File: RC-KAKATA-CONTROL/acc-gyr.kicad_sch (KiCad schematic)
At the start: 10 parts, among them U13 ICM-20689

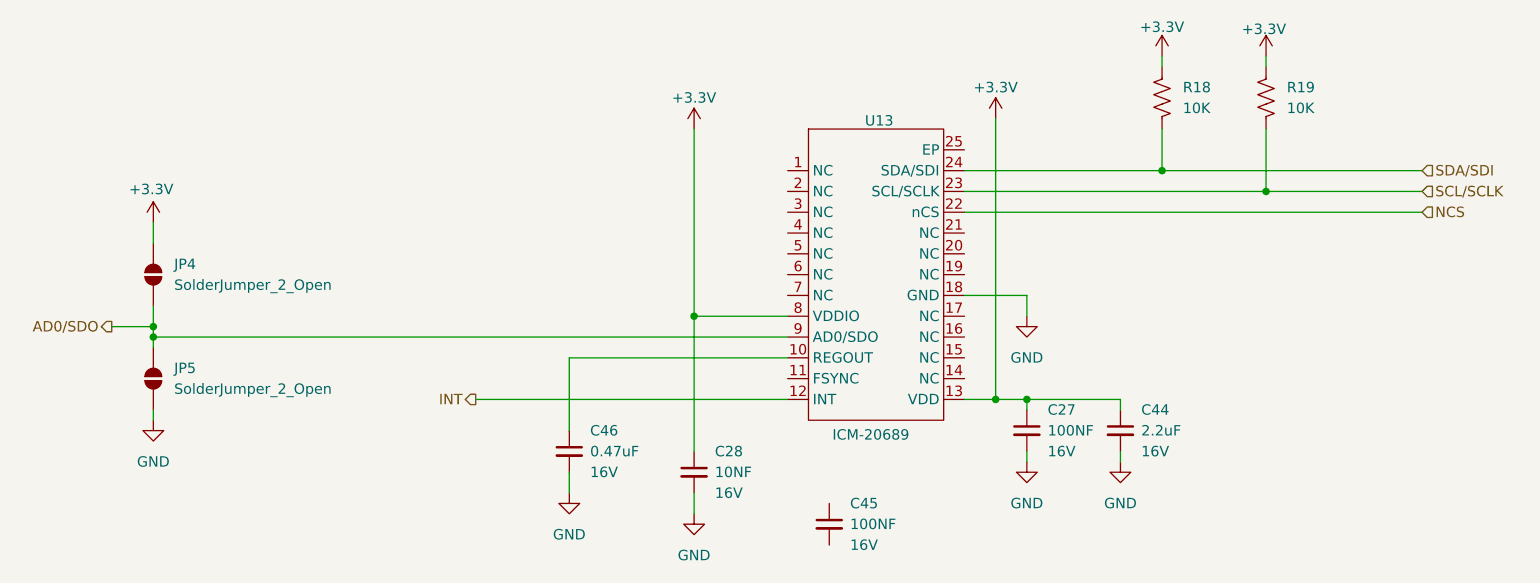
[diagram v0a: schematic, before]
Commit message: Agregadas conexiones de analogicos Agregadas las conexiones de i2c Agregadas las conexiones de Uart Cambiados algunos detalles de tvs resistencias y cap Recolocados los componenetes de power supply Cambiados los diodos de entrada de la bateria por unos de 5A Cambios menores y mejorada la documentacion Agregada informacion en la serigrafia del PCB
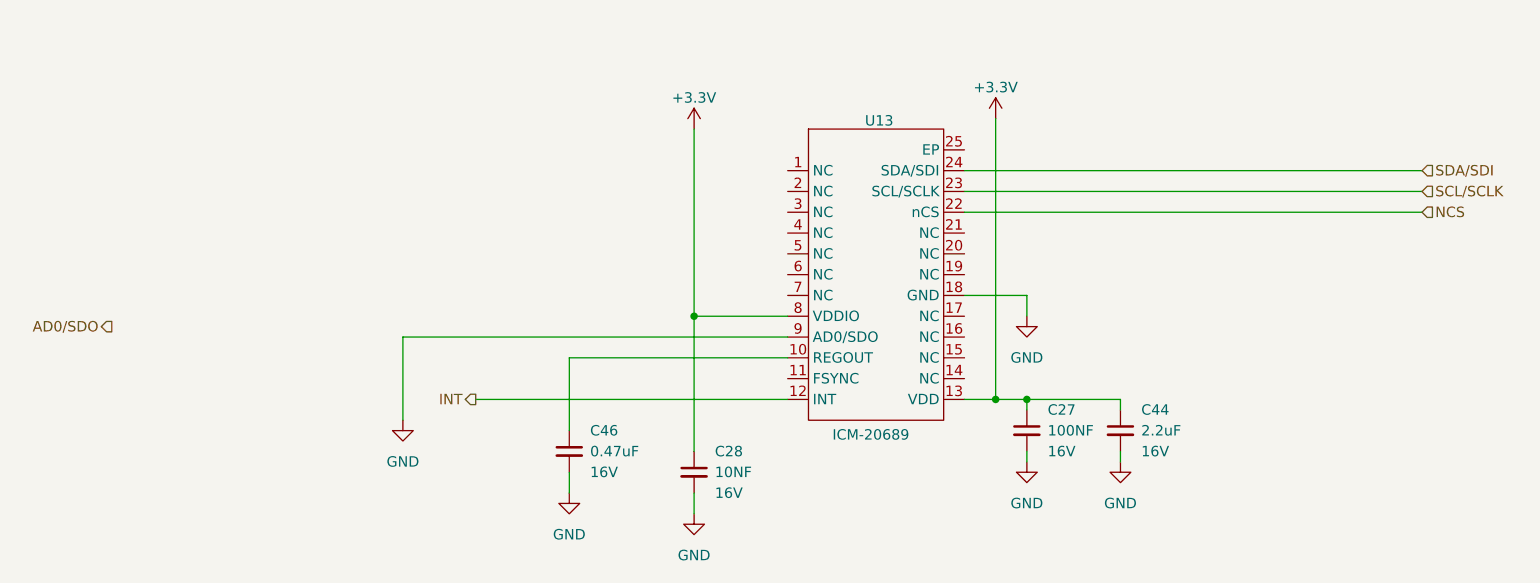
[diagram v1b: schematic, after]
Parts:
- removed C45: 100NF, 4ms_Capacitor:C_0603, symbol MG_CAPACITOR:CAP-0603-100NF-16V-X5R
- removed JP4, JP5: SolderJumper_2_Open, 4ms_SolderJumper:JUMPER_SMD_1x2, symbol Jumper:SolderJumper_2_Open
- removed R18, R19: 10K, 4ms_Resistor:R_0603, symbol MG_RESISTOR:RES-0603-10K-1%
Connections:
- net AD0/SDO: no longer U13.9 (AD0/SDO)
- net GND: now also U13.9 (AD0/SDO)
